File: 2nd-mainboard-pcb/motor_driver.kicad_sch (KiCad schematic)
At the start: 15 parts, among them J10 Servo Motor BL Touch, J11 T3, J7 Stepper Motor, J8 Servo Motor SM, J9 Microstepping, U12 MPU-6050

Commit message: motor module traced
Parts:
- C28: footprint Capacitor_SMD:C_0603_1608Metric_Pad1.08x0.95mm_HandSolder -> Capacitor_SMD:C_0805_2012Metric_Pad1.18x1.45mm_HandSolder
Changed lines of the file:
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@@
 			)
 		)
-		(property "Footprint" "Capacitor_SMD:C_0603_1608Metric_Pad1.08x0.95mm_HandSolder"
+		(property "Footprint" "Capacitor_SMD:C_0805_2012Metric_Pad1.18x1.45mm_HandSolder"
 			(at 33.9852 156.21 0)
 			(effects

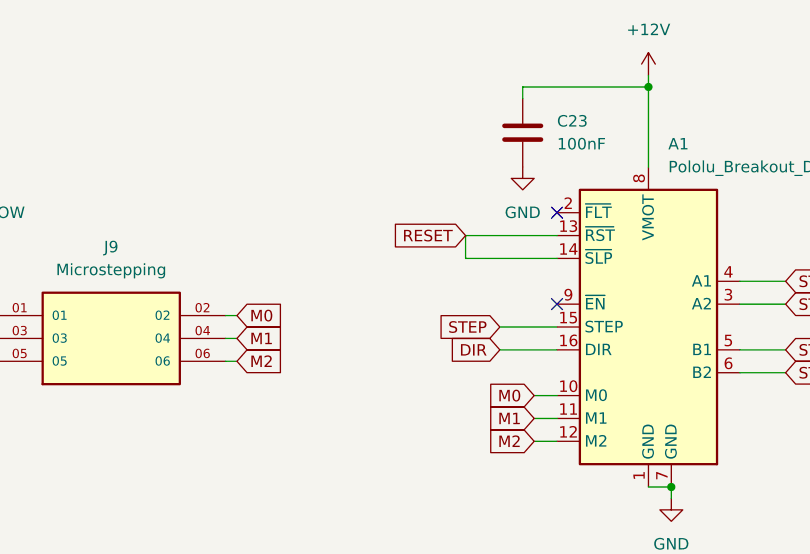
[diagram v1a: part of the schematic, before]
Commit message: last few changes
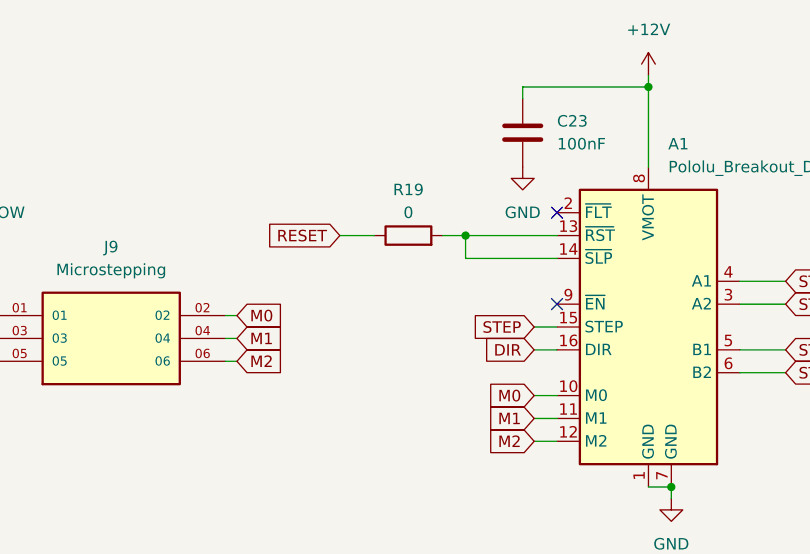
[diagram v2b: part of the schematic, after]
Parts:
- added R19: 0, Resistor_SMD:R_0603_1608Metric_Pad0.98x0.95mm_HandSolder, symbol Device:R
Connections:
- net RESET: now also R19.1; no longer A1.13 (~{RST}), A1.14 (~{SLP})
- new net: A1.13 (~{RST}), A1.14 (~{SLP}), R19.2
